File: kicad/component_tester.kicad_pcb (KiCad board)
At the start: 2 copper layers, 100.4 x 83 mm, 81 parts, among them IC201 MCP1640, IC202 ATmega328P-MMH, IC301 FT232RL, IC302 MAX1811, J301 0R-JUMPA, J302 0R-JUMPA, Q201 8 MHz, Q401 BSS138, Q402 BSS138, SW201 EVQ, T201 PMV65XP, T202 BSS84, T203 BSS123, T204 BC847, T301 BSS123, X201 MICRO-USB, X202 ISP

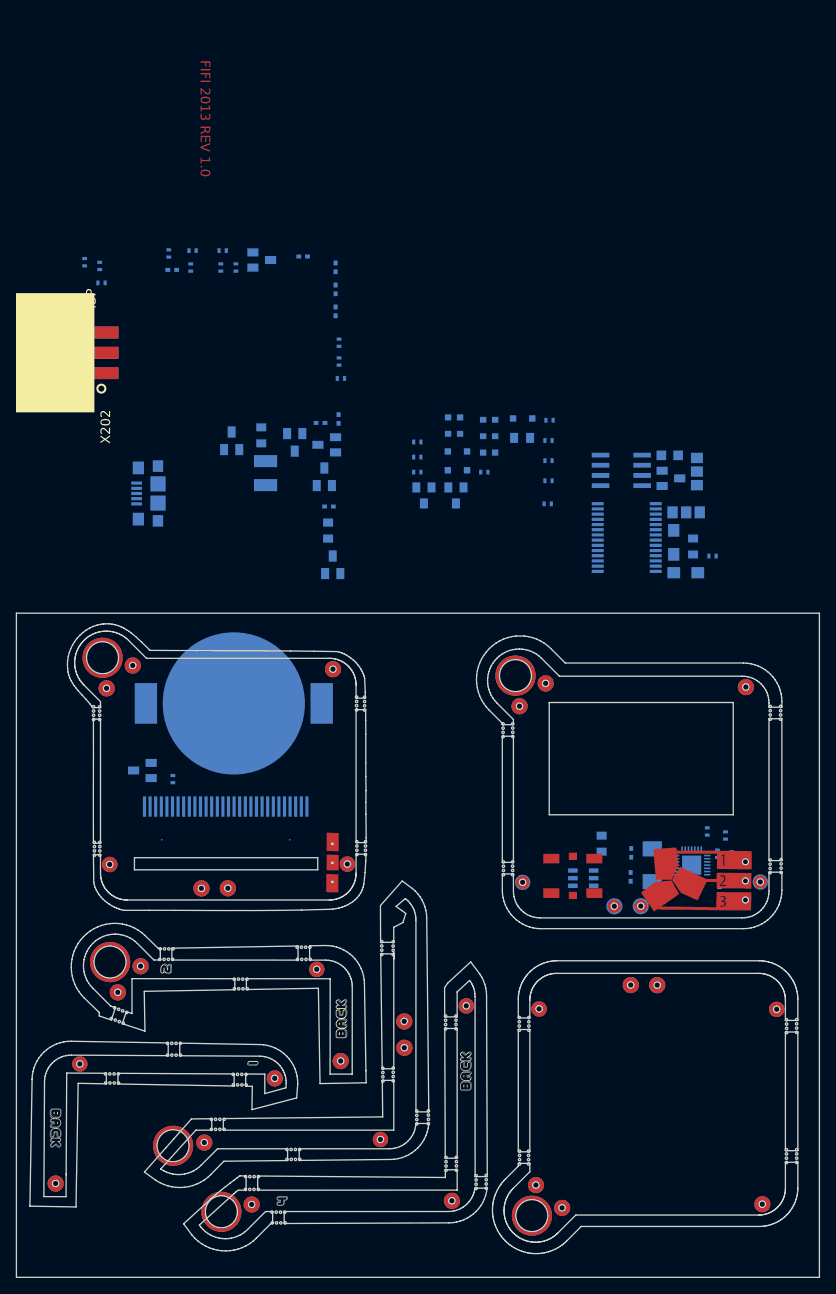
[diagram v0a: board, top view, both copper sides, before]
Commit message: Work on placing components
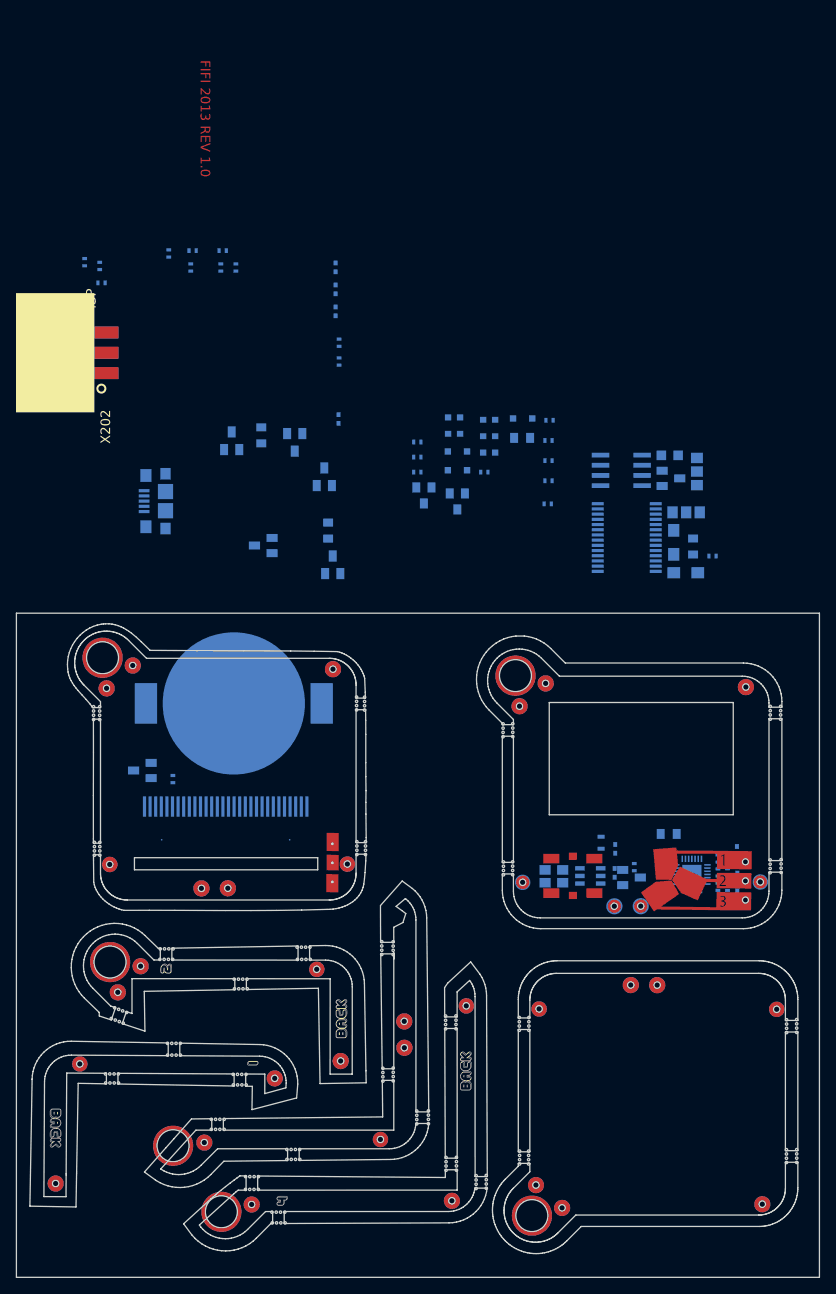
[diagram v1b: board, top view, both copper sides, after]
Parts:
- L201: value 4,7 uH -> 4.7uH; footprint component_tester:L1210 -> KiCad/Resistors_SMD.pretty:R_0603
- Q201: footprint KiCad/Crystals.pretty:Crystal_SMD_Abracon_ABM3-2pin_5.0x3.2mm -> mcous/kicad-lib/footprints/crystal.pretty:NDK-NX3225GA_xtal
- moved C202 96.6 mm to (170.8, 108.2), turned to 270 degrees
- moved C209 92.0 mm to (179.7, 106.3), turned to 270 degrees
- moved T202 90.0 mm to (166.6, 109.7)
- moved C208 76.3 mm to (179.8, 108.5), turned to 270 degrees
- moved R206 71.2 mm to (166.9, 108.3), turned to 270 degrees
- moved C210 69.7 mm to (179.8, 110.7), turned to 90 degrees
- moved L201 62.4 mm to (162.8, 105.3)
- moved D202 14.9 mm to (120.5, 68.2)
- moved Q201 12.4 mm to (156.8, 109.5), turned to 270 degrees
- moved C201 8.47 mm to (171.2, 104.2), turned to 0 degrees
- moved R216 3.64 mm to (177.4, 107.3), turned to 270 degrees
- moved R215 2.87 mm to (178.6, 107.2), turned to 270 degrees
- moved R214 2.73 mm to (177.4, 109.0)
- moved R217 2.64 mm to (178.6, 109.0)
- moved C204 2.06 mm to (164.5, 106.1)
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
